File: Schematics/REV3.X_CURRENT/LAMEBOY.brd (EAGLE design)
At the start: 45.7 x 67.3 mm, 64 parts, among them IC1 PCF8574T, IC3 MCP73831, Q1 12MHz, U1 USD-SOCKETMICROSDEBAY

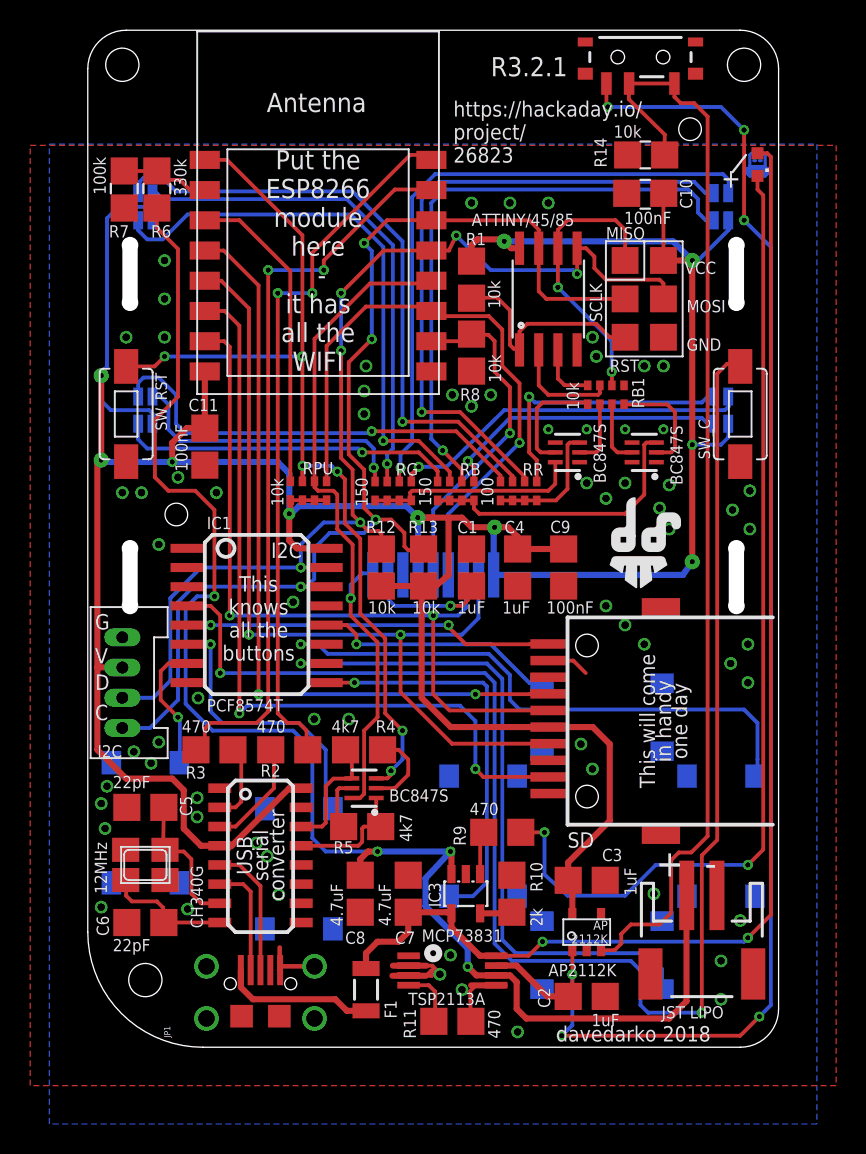
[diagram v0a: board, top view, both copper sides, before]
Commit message: minor footprint changes
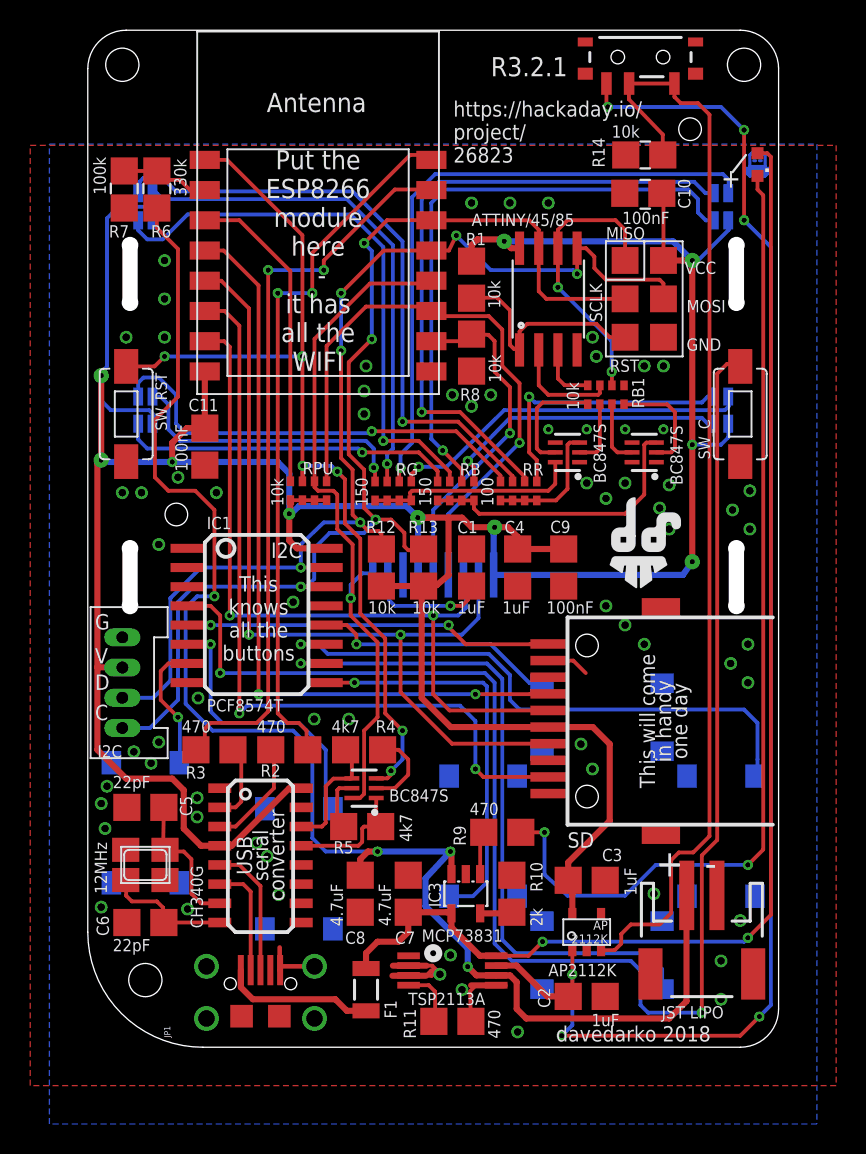
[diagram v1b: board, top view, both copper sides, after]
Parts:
- moved C10 0.13 mm to (36.8, 56.5)
- moved R14 0.13 mm to (36.8, 59.1)
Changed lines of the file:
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@@
 <layers>
 <layer number="1" name="Top" color="4" fill="1" visible="yes" active="yes"/>
-<layer number="16" name="Bottom" color="1" fill="1" visible="no" active="yes"/>
+<layer number="16" name="Bottom" color="1" fill="1" visible="yes" active="yes"/>
 <layer number="17" name="Pads" color="2" fill="1" visible="yes" active="yes"/>
 <layer number="18" name="Vias" color="2" fill="1" visible="yes" active="yes"/>
@@
 <layer number="20" name="Dimension" color="15" fill="1" visible="yes" active="yes"/>
 <layer number="21" name="tPlace" color="7" fill="1" visible="yes" active="yes"/>
-<layer number="22" name="bPlace" color="7" fill="1" visible="no" active="yes"/>
+<layer number="22" name="bPlace" color="7" fill="1" visible="yes" active="yes"/>
 <layer number="23" name="tOrigins" color="15" fill="1" visible="yes" active="yes"/>
-<layer number="24" name="bOrigins" color="15" fill="1" visible="no" active="yes"/>
+<layer number="24" name="bOrigins" color="15" fill="1" visible="yes" active="yes"/>
 <layer number="25" name="tNames" color="7" fill="1" visible="yes" active="yes"/>
 <layer number="26" name="bNames" color="7" fill="1" visible="yes" active="yes"/>
-<layer number="27" name="tValues" color="7" fill="1" visible="no" active="yes"/>
-<layer number="28" name="bValues" color="7" fill="1" visible="no" active="yes"/>
+<layer number="27" name="tValues" color="7" fill="1" visible="yes" active="yes"/>
+<layer number="28" name="bValues" color="7" fill="1" visible="yes" active="yes"/>
 <layer number="29" name="tStop" color="7" fill="3" visible="no" active="yes"/>
 <layer number="30" name="bStop" color="7" fill="6" visible="no" active="yes"/>
@@
 <attribute name="VALUE" x="30.353" y="28.702" size="0.8128" layer="25" ratio="12"/>
 </element>
-<element name="C10" library="rcl" package="ONEFITSALL" value="100nF" x="36.8935" y="56.515" smashed="yes">
-<attribute name="NAME" x="40.005" y="55.499" size="0.8128" layer="25" ratio="12" rot="R90"/>
-<attribute name="VALUE" x="35.4965" y="54.483" size="0.8128" layer="25" ratio="12"/>
+<element name="C10" library="rcl" package="ONEFITSALL" value="100nF" x="36.7665" y="56.515" smashed="yes">
+<attribute name="NAME" x="39.878" y="55.499" size="0.8128" layer="25" ratio="12" rot="R90"/>
+<attribute name="VALUE" x="35.3695" y="54.483" size="0.8128" layer="25" ratio="12"/>
 </element>
 <element name="C11" library="rcl" package="ONEFITSALL" value="100nF" x="7.747" y="39.751" smashed="yes" rot="R90">
@@
 <element name="U$13" library="LOGOS" package="DAVEDARKO_GOLD" value="" x="34.036" y="12.827" rot="MR0"/>
 <element name="JP1" library="SparkFun-Connectors" package="USB-AB-MICRO-SMD_SLOT" value="USB_MICROB_PLUG-IDK" x="11.43" y="1.905" rot="R90"/>
-<element name="R14" library="rcl" package="ONEFITSALL" value="10k" x="36.957" y="59.055" smashed="yes" rot="R180">
-<attribute name="NAME" x="33.528" y="60.198" size="0.8128" layer="25" ratio="12" rot="R270"/>
-<attribute name="VALUE" x="34.798" y="60.198" size="0.8128" layer="25" ratio="12"/>
+<element name="R14" library="rcl" package="ONEFITSALL" value="10k" x="36.83" y="59.055" smashed="yes" rot="R180">
+<attribute name="NAME" x="33.401" y="60.198" size="0.8128" layer="25" ratio="12" rot="R270"/>
+<attribute name="VALUE" x="34.671" y="60.198" size="0.8128" layer="25" ratio="12"/>
 </element>
 </elements>
@@
 <contactref element="C11" pad="P$2"/>
 <wire x1="38.1" y1="52.07" x2="38.1" y2="57.1475" width="0.254" layer="1"/>
-<wire x1="38.1" y1="57.1475" x2="38.1185" y2="56.515" width="0.254" layer="1"/>
-<wire x1="38.1" y1="57.1525" x2="38.1185" y2="56.515" width="0.254" layer="1"/>
+<wire x1="38.1" y1="57.1475" x2="37.9915" y2="56.515" width="0.254" layer="1"/>
+<wire x1="38.1" y1="57.1525" x2="37.9915" y2="56.515" width="0.254" layer="1"/>
 <wire x1="27.527" y1="53.372" x2="27.559" y2="53.34" width="0.4064" layer="1"/>
 <wire x1="31.496" y1="32.975" x2="28.448" y2="32.975" width="0.4064" layer="1"/>
@@
 <wire x1="35.826" y1="63.782" x2="38.826" y2="63.782" width="0.254" layer="1"/>
 <wire x1="38.608" y1="12.3825" x2="39.116" y2="12.8905" width="0.254" layer="1"/>
-<wire x1="39.116" y1="12.8905" x2="39.9415" y2="12.8905" width="0.254" layer="1"/>
-<wire x1="39.9415" y1="12.8905" x2="41.021" y2="13.97" width="0.254" layer="1"/>
-<wire x1="41.021" y1="13.97" x2="41.021" y2="61.595" width="0.254" layer="1"/>
-<wire x1="41.021" y1="61.595" x2="40.132" y2="62.484" width="0.254" layer="1"/>
+<wire x1="39.116" y1="12.8905" x2="40.0685" y2="12.8905" width="0.254" layer="1"/>
+<wire x1="40.0685" y1="12.8905" x2="41.148" y2="13.97" width="0.254" layer="1"/>
+<wire x1="41.148" y1="13.97" x2="41.148" y2="61.722" width="0.254" layer="1"/>
+<wire x1="41.148" y1="61.722" x2="40.386" y2="62.484" width="0.254" layer="1"/>
 <wire x1="33.97" y1="6.42" x2="34.868" y2="6.42" width="0.254" layer="1"/>
 <wire x1="34.868" y1="6.42" x2="35.306" y2="6.858" width="0.254" layer="1"/>
@@
 <wire x1="38.608" y1="8.89" x2="38.608" y2="12.3825" width="0.254" layer="1"/>
 <contactref element="R14" pad="P$1"/>
-<wire x1="40.132" y1="62.484" x2="39.243" y2="62.484" width="0.254" layer="1"/>
+<wire x1="40.386" y1="62.484" x2="39.243" y2="62.484" width="0.254" layer="1"/>
 <wire x1="39.243" y1="62.484" x2="38.826" y2="62.901" width="0.254" layer="1"/>
 <wire x1="38.826" y1="63.782" x2="38.826" y2="62.901" width="0.254" layer="1"/>
-<wire x1="38.182" y1="59.055" x2="38.182" y2="60.407" width="0.254" layer="1"/>
-<wire x1="38.182" y1="60.407" x2="35.814" y2="62.738" width="0.254" layer="1"/>
+<wire x1="38.055" y1="59.055" x2="38.055" y2="60.407" width="0.254" layer="1"/>
+<wire x1="38.055" y1="60.407" x2="35.814" y2="62.738" width="0.254" layer="1"/>
 <wire x1="35.814" y1="62.738" x2="35.814" y2="63.77" width="0.254" layer="1"/>
 <wire x1="35.814" y1="63.77" x2="35.826" y2="63.782" width="0.254" layer="1"/>
